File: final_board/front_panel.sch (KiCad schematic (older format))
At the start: 10 parts, among them P100 ISP, P101 DEBUG_LED

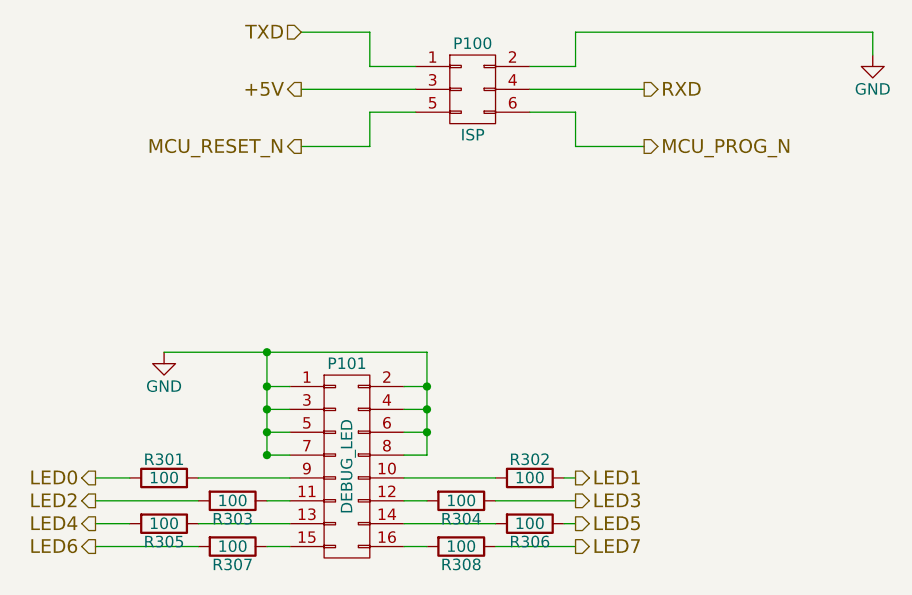
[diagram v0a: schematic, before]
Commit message: Final changes to board
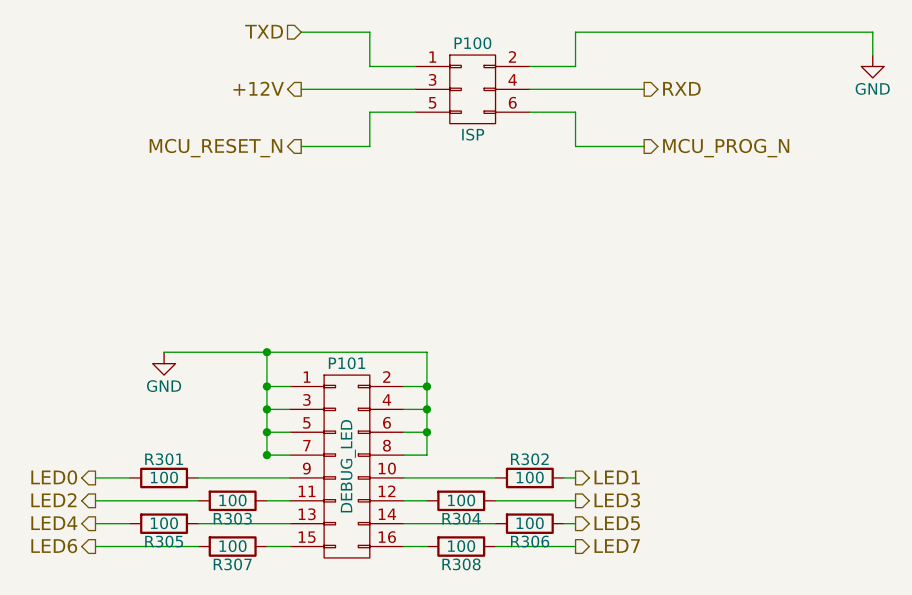
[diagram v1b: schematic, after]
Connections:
- net +5V renamed +12V
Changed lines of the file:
@@
 EESchema Schematic File Version 2
-LIBS:final_outline-rescue
 LIBS:power
 LIBS:device
@@
 LIBS:MITEVT_power
 LIBS:MITEVT_REG
+LIBS:zsr1000gta
 LIBS:final_outline-cache
 EELAYER 25 0
@@
 $EndComp
 Text HLabel 2800 2050 0    60   Output ~ 0
-+5V
++12V
 Text HLabel 4300 2050 2    60   Output ~ 0
 RXD
@@
 MCU_PROG_N
 $Comp
-L GND #PWR06
+L GND #PWR07
 U 1 1 563E4869
 P 5300 1900
-F 0 "#PWR06" H 5300 1650 50  0001 C CNN
+F 0 "#PWR07" H 5300 1650 50  0001 C CNN
 F 1 "GND" H 5300 1750 50  0000 C CNN
 F 2 "" H 5300 1900 60  0000 C CNN
@@
 LED1
 $Comp
-L GND #PWR07
+L GND #PWR08
 U 1 1 563E4469
 P 2200 3200
-F 0 "#PWR07" H 2200 2950 50  0001 C CNN
+F 0 "#PWR08" H 2200 2950 50  0001 C CNN
 F 1 "GND" H 2200 3050 50  0000 C CNN
 F 2 "" H 2200 3200 60  0000 C CNN

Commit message: Fixed some routing
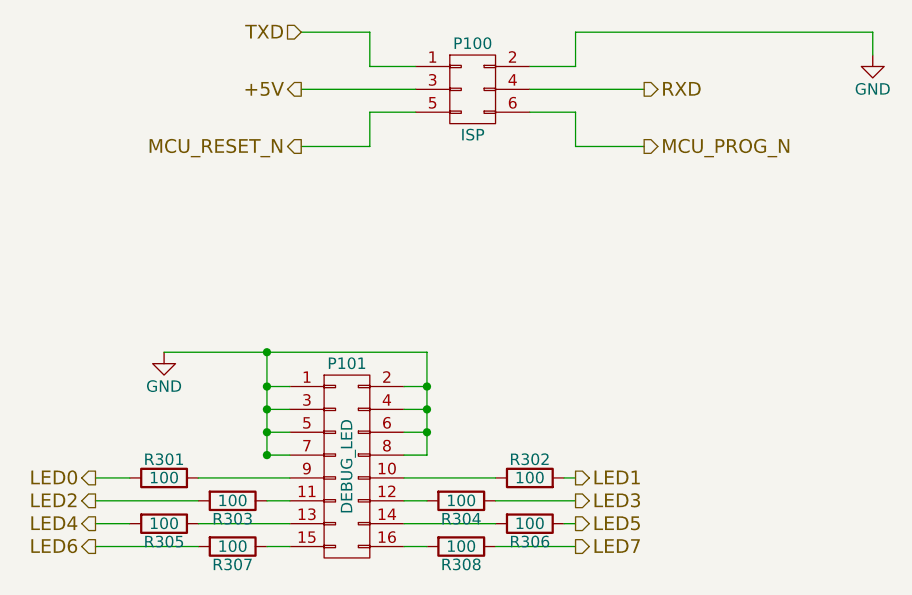
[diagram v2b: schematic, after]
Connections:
- net +12V renamed +5V
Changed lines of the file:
@@
 LIBS:MITEVT_power
 LIBS:MITEVT_REG
-LIBS:zsr1000gta
 LIBS:final_outline-cache
 EELAYER 25 0
@@
 $EndComp
 Text HLabel 2800 2050 0    60   Output ~ 0
-+12V
++5V
 Text HLabel 4300 2050 2    60   Output ~ 0
 RXD
